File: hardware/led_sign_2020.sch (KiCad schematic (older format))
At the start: 29 parts, among them U1 ESP32-DevKitC, U2 MC74VHC1GT125, U3 MC74VHC1GT125, U4 MAX17601, U5 MAX17601, U6 MAX17601, U7 MAX17601

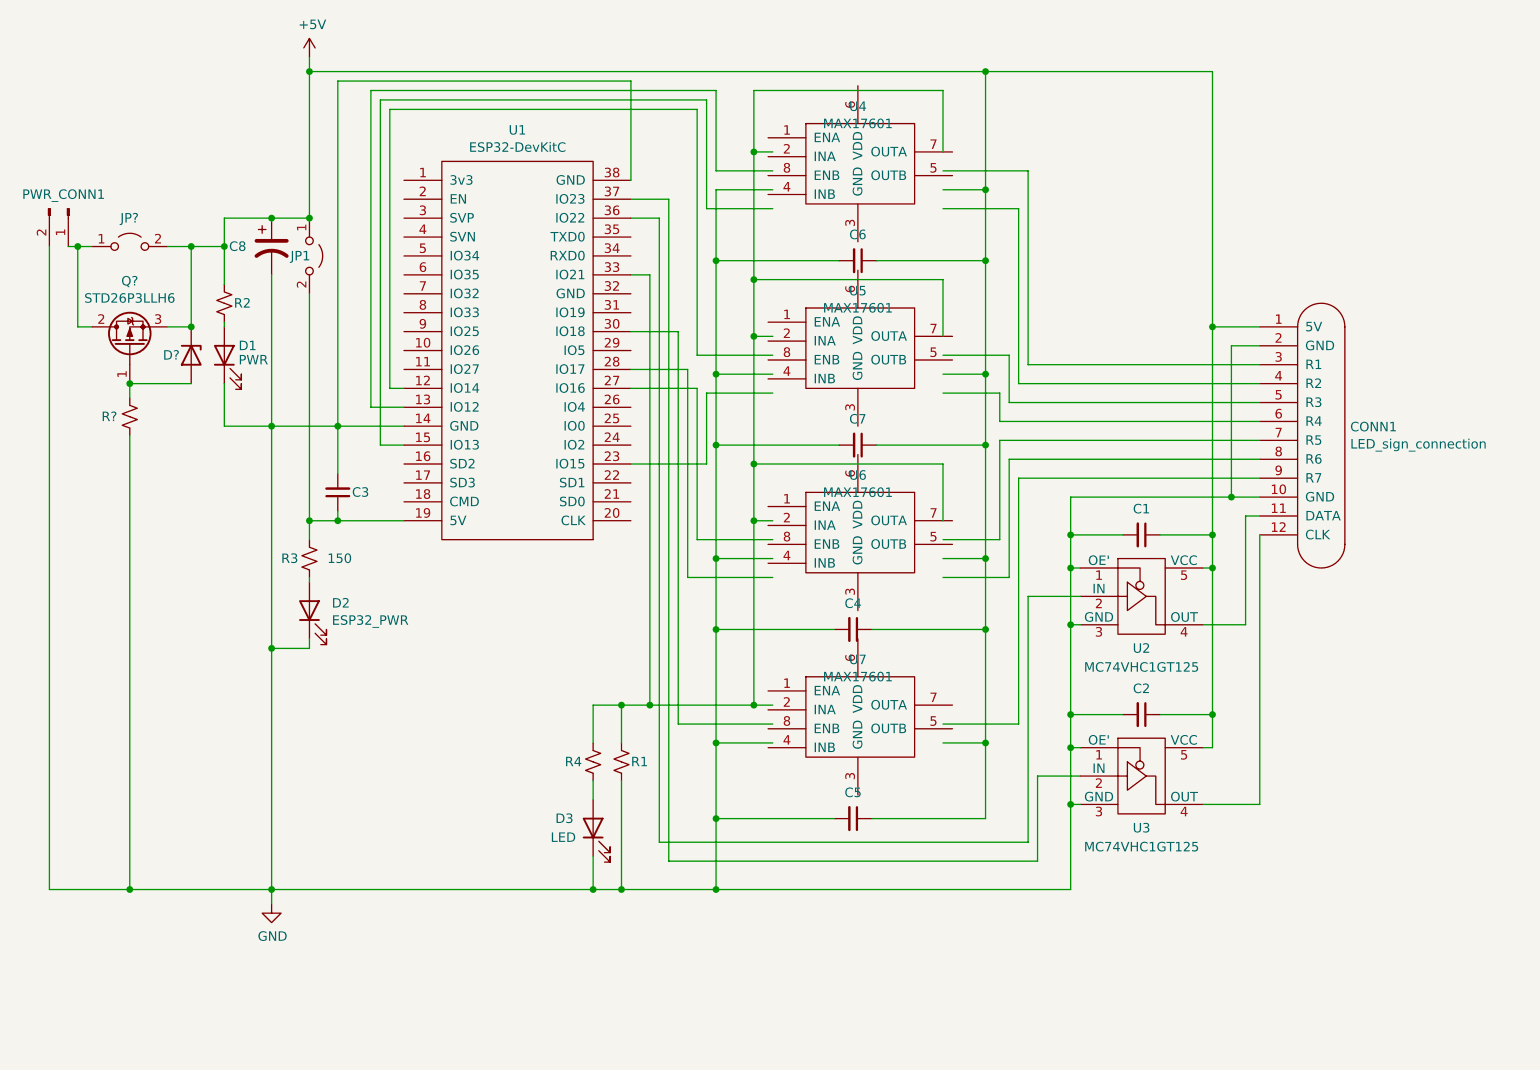
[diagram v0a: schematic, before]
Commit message: all kinds of reorg and netlabels
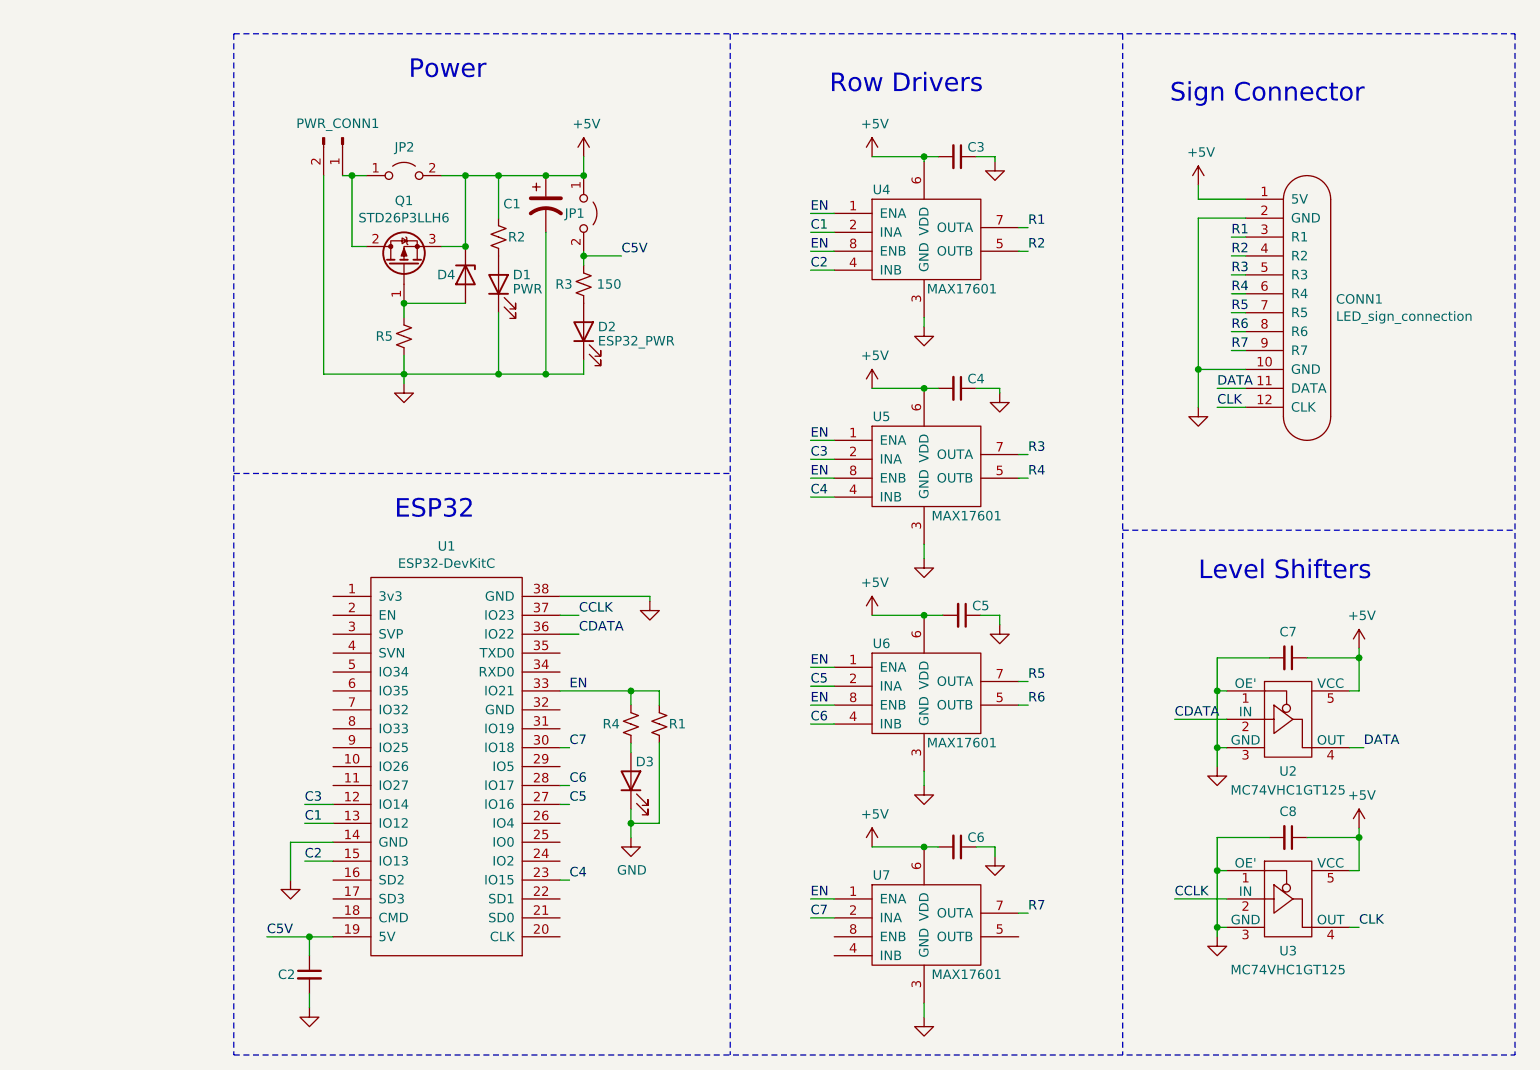
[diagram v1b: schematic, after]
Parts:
- removed C5: 0.1uF, Capacitor_SMD:C_0805_2012Metric, symbol Device:C_Small
- added C3: 0.1uF, Capacitor_SMD:C_0805_2012Metric, symbol Device:C_Small
- Q1: renamed from Q?; footprint Package_TO_SOT_SMD:TO-252-2 -> Package_TO_SOT_SMD:TO-252-3_TabPin2
- gave numbers to parts that had none: 3
- renumbered C8 to C1, C3 to C2, C6 to C4, C7 to C5, C4 to C6, C1 to C7, C2 to C8
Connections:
- net labels added: C1, C2, C3, C4, C5, C5V, C6, C7, CCLK, CDATA, CLK, DATA, EN, R1, R2, R3, R4, R5, R6, R7
- wire segments 195 -> 134
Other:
- note added: "ESP32"
- note added: "Level Shifters"
- note added: "Power"
- note added: "Row Drivers"
- note added: "Sign Connector"
- moved on the sheet: C1, C2, C4, C5, C6, C7, C8, CONN1, D1, D2, D3, D4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

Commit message: associate footprint
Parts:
- D4: footprint (none) -> Diode_SMD:D_0805_2012Metric
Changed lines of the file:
@@
 F 0 "D4" V 3225 2100 50  0000 L CNN
 F 1 "D_Zener" V 3270 2330 50  0001 L CNN
-F 2 "" H 3225 2250 50  0001 C CNN
+F 2 "Diode_SMD:D_0805_2012Metric" H 3225 2250 50  0001 C CNN
 F 3 "~" H 3225 2250 50  0001 C CNN
 	1    3225 2250

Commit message: routing pcb
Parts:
- C1: footprint (none) -> Capacitor_THT:CP_Radial_D10.0mm_P5.00mm
- CONN1: footprint (none) -> Connector_JST:JST_XH_B12B-XH-A_1x12_P2.50mm_Vertical
- JP1: value Jumper_2_Open -> ESP32_5V
- JP2: value Jumper_2_Open -> prot_short
- PWR_CONN1: footprint (none) -> Connector_JST:JST_XH_B2B-XH-A_1x02_P2.50mm_Vertical
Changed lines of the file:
@@
 F 0 "PWR_CONN1" V 2500 1500 50  0000 C CNN
 F 1 "Conn_01x02_Male" H 2683 1615 50  0001 C CNN
-F 2 "" H 2575 1525 50  0001 C CNN
+F 2 "Connector_JST:JST_XH_B2B-XH-A_1x02_P2.50mm_Vertical" H 2575 1525 50  0001 C CNN
 F 3 "~" H 2575 1525 50  0001 C CNN
 	1    2575 1525
@@
 F 0 "CONN1" H 7828 1021 50  0000 L CNN
 F 1 "LED_sign_connection" H 7828 930 50  0000 L CNN
-F 2 "" H 7350 1700 50  0001 C CNN
+F 2 "Connector_JST:JST_XH_B12B-XH-A_1x12_P2.50mm_Vertical" H 7350 1700 50  0001 C CNN
 F 3 "" H 7350 1700 50  0001 C CNN
 	1    7350 1700
@@
 F 0 "C1" H 3425 1875 50  0000 L CNN
 F 1 "CP1" H 3400 1875 50  0001 L CNN
-F 2 "" H 3650 1875 50  0001 C CNN
+F 2 "Capacitor_THT:CP_Radial_D10.0mm_P5.00mm" H 3650 1875 50  0001 C CNN
 F 3 "~" H 3650 1875 50  0001 C CNN
 	1    3650 1875
@@
 P 2900 1725
 F 0 "JP2" H 2850 1875 50  0000 L CNN
-F 1 "Jumper_2_Open" H 2900 1869 50  0001 C CNN
+F 1 "prot_short" H 2900 1869 50  0001 C CNN
 F 2 "Connector_PinHeader_2.54mm:PinHeader_1x02_P2.54mm_Vertical" H 2900 1725 50  0001 C CNN
 F 3 "~" H 2900 1725 50  0001 C CNN
@@
 P 3850 1925
 F 0 "JP1" V 3850 1825 50  0000 L CNN
-F 1 "Jumper_2_Open" H 3850 2069 50  0001 C CNN
+F 1 "ESP32_5V" H 3850 2069 50  0001 C CNN
 F 2 "Connector_PinHeader_2.54mm:PinHeader_1x02_P2.54mm_Vertical" H 3850 1925 50  0001 C CNN
 F 3 "~" H 3850 1925 50  0001 C CNN
